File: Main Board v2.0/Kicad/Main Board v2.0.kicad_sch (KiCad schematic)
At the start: 0 parts

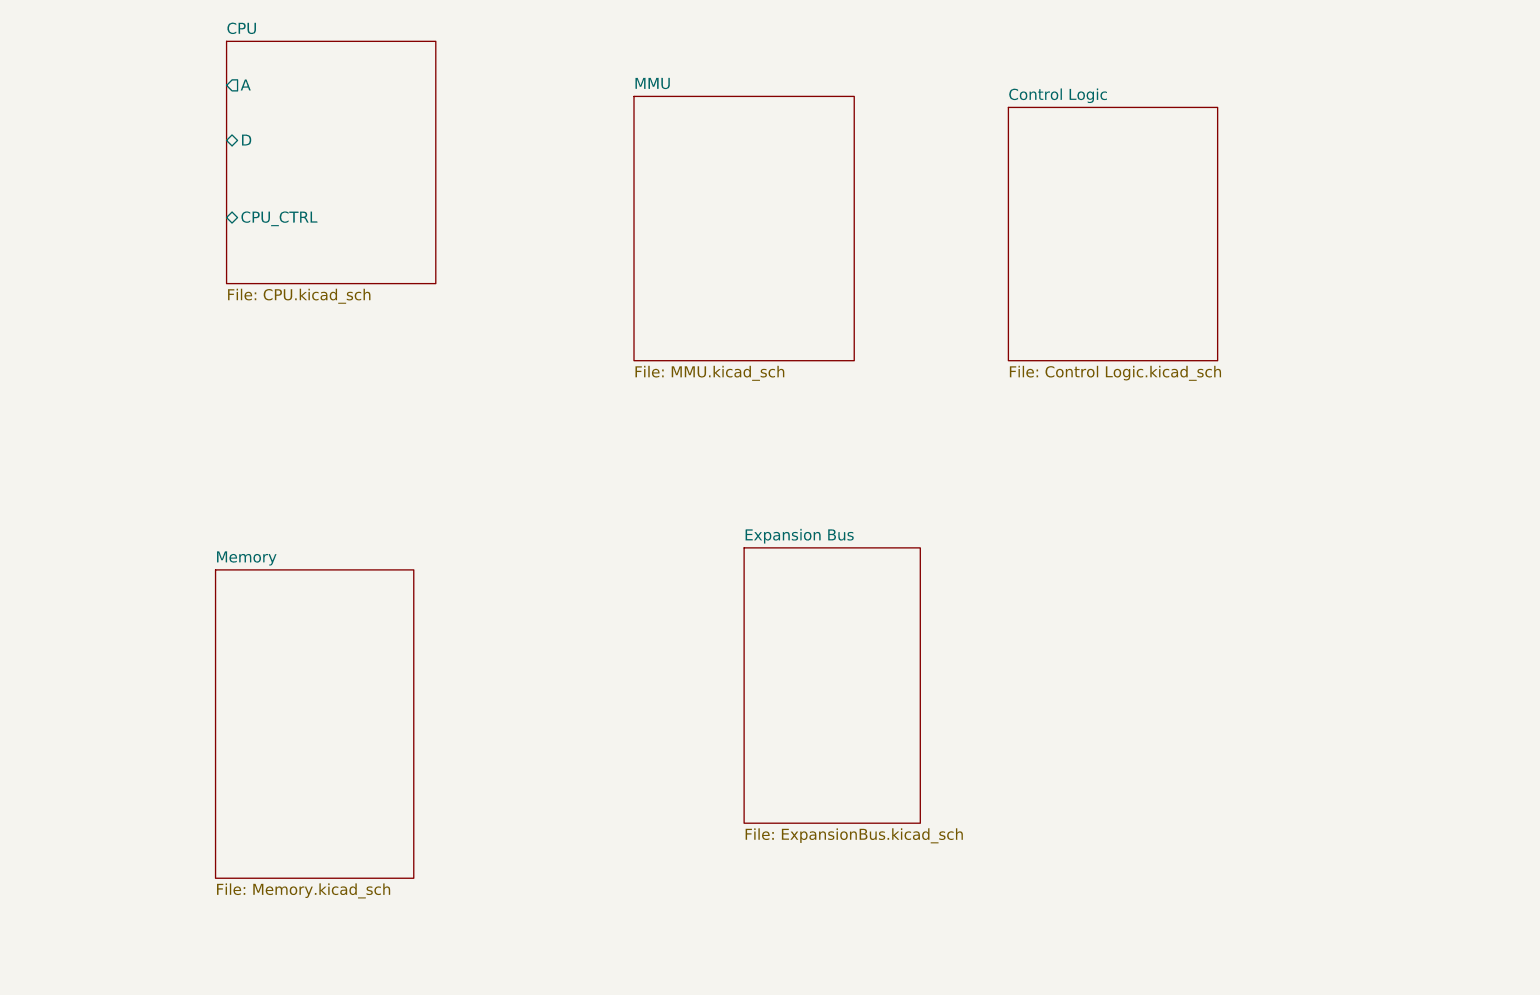
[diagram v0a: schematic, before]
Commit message: update
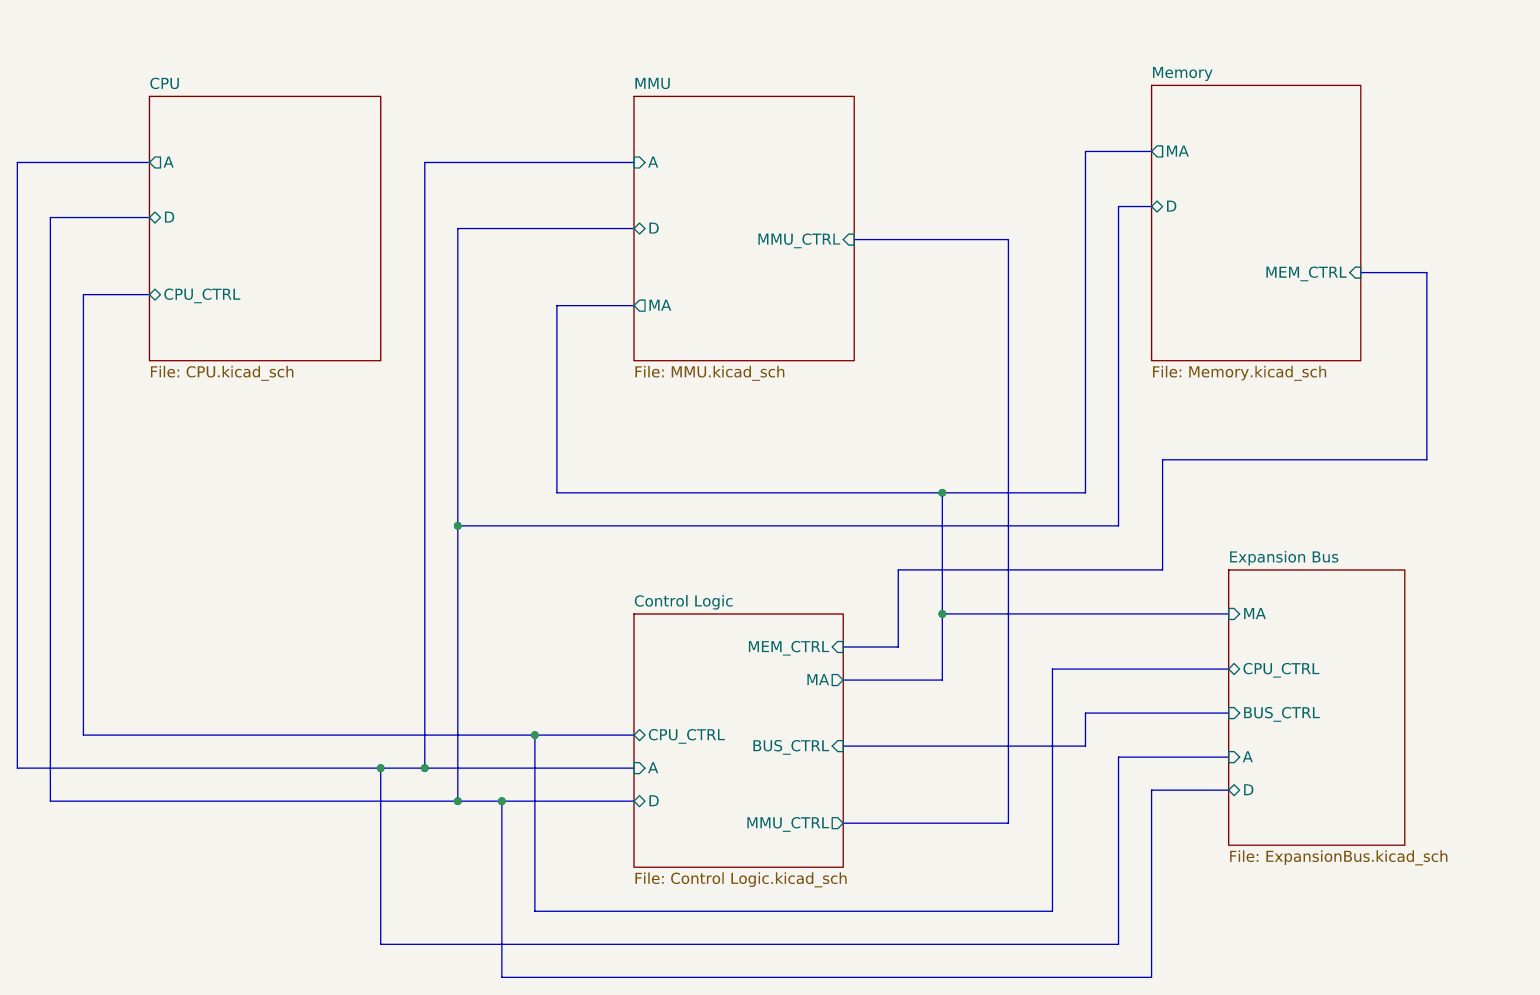
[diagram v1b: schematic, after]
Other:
- sheet Control Logic ports: added A, BUS_CTRL, CPU_CTRL, D, MA, MEM_CTRL, MMU_CTRL; removed none
- sheet Expansion Bus ports: added A, BUS_CTRL, CPU_CTRL, D, MA; removed none
- sheet MMU ports: added A, D, MA, MMU_CTRL; removed none
- sheet Memory ports: added D, MA, MEM_CTRL; removed none

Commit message: schematic done*
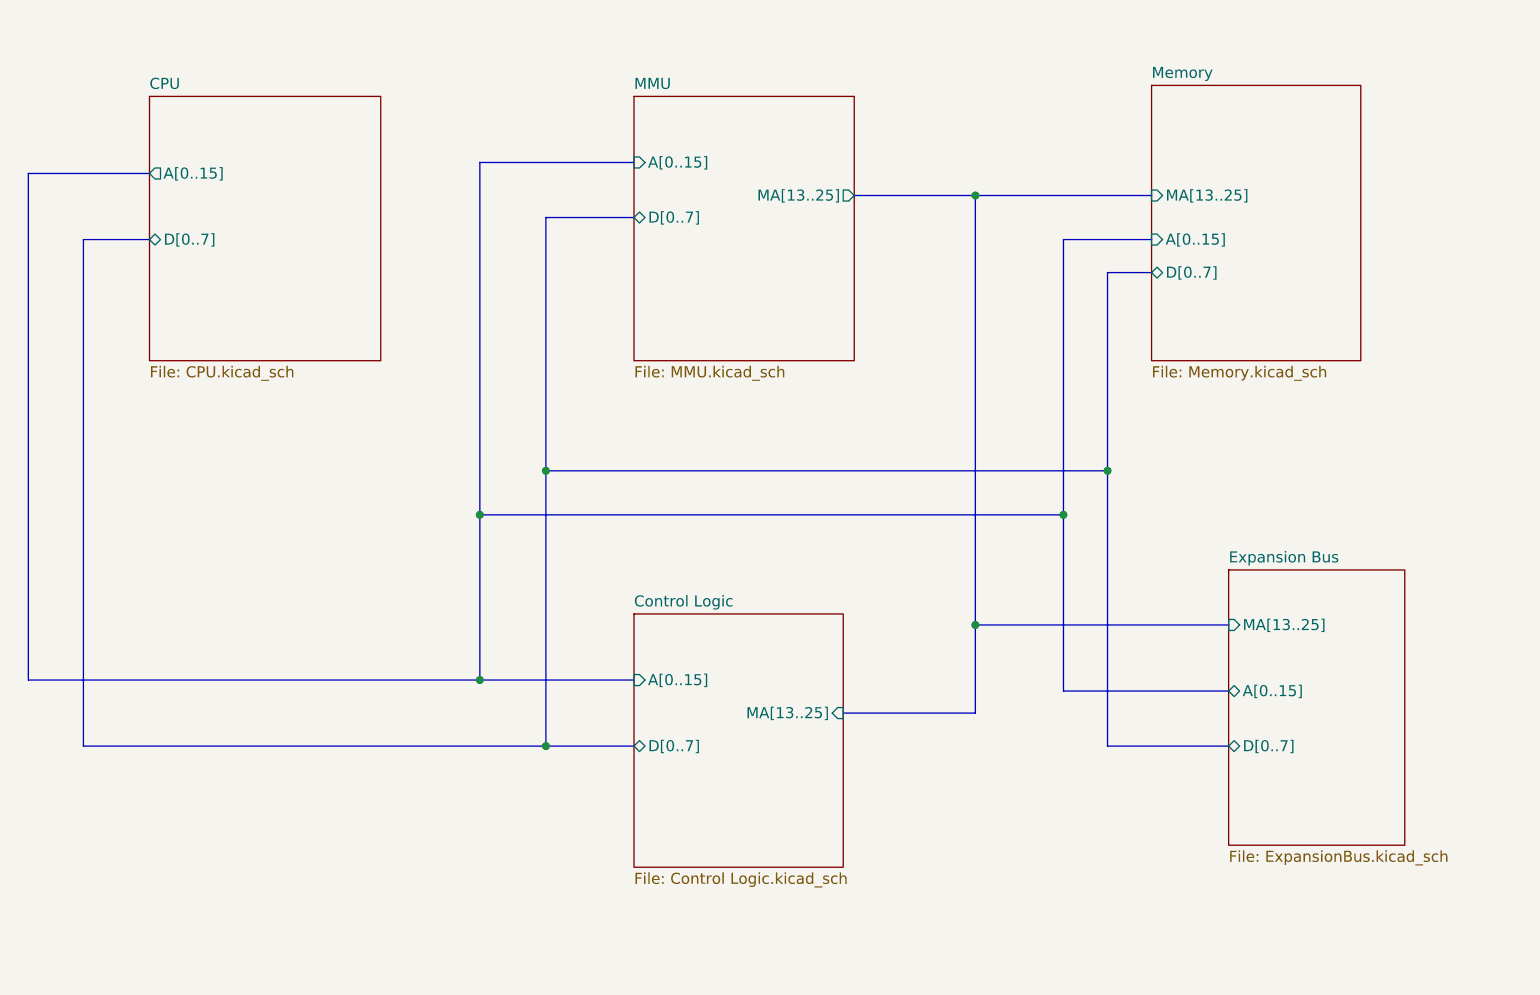
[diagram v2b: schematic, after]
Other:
- sheet CPU ports: added A[0..15], D[0..7]; removed A, CPU_CTRL, D
- sheet Control Logic ports: added A[0..15], D[0..7], MA[13..25]; removed A, BUS_CTRL, CPU_CTRL, D, MA, MEM_CTRL, MMU_CTRL
- sheet Expansion Bus ports: added A[0..15], D[0..7], MA[13..25]; removed A, BUS_CTRL, CPU_CTRL, D, MA
- sheet MMU ports: added A[0..15], D[0..7], MA[13..25]; removed A, D, MA, MMU_CTRL
- sheet Memory ports: added A[0..15], D[0..7], MA[13..25]; removed D, MA, MEM_CTRL
